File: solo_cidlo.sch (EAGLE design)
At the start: 4 parts, among them Q1 QRD1114

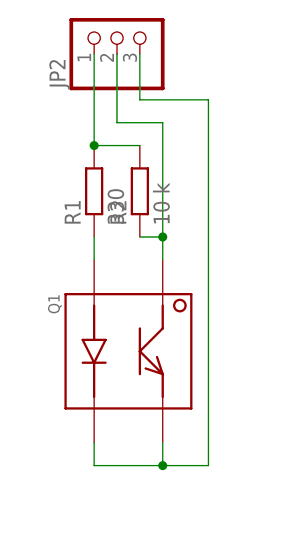
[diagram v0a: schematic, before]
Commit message: Add files via upload
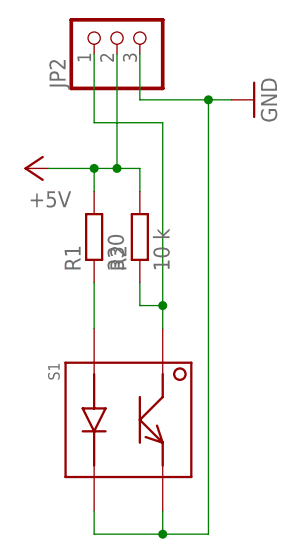
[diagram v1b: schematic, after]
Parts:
- removed Q1: QRD1114, QRD1114:QRD1114
- added S1: QRD1114, QRD1114:QRD1114
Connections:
- removed net N$3: JP2.1, R1.2, R2.2
- removed net N$4: JP2.3, Q1.P$2, Q1.P$4
- new net +5V: JP2.2, R1.2, R2.2
- new net GND: JP2.3, S1.P$2, S1.P$4
- net N$1: now also S1.P$3; no longer Q1.P$3
- net N$2: now also JP2.1, S1.P$1; no longer JP2.2, Q1.P$1
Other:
- moved on the sheet: R1, R2
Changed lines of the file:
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@@
 <layers>
 <layer number="1" name="Top" color="4" fill="1" visible="no" active="no"/>
+<layer number="2" name="Route2" color="1" fill="3" visible="no" active="no"/>
+<layer number="3" name="Route3" color="4" fill="3" visible="no" active="no"/>
+<layer number="4" name="Route4" color="1" fill="4" visible="no" active="no"/>
+<layer number="5" name="Route5" color="4" fill="4" visible="no" active="no"/>
+<layer number="6" name="Route6" color="1" fill="8" visible="no" active="no"/>
+<layer number="7" name="Route7" color="4" fill="8" visible="no" active="no"/>
+<layer number="8" name="Route8" color="1" fill="2" visible="no" active="no"/>
+<layer number="9" name="Route9" color="4" fill="2" visible="no" active="no"/>
+<layer number="10" name="Route10" color="1" fill="7" visible="no" active="no"/>
+<layer number="11" name="Route11" color="4" fill="7" visible="no" active="no"/>
+<layer number="12" name="Route12" color="1" fill="5" visible="no" active="no"/>
+<layer number="13" name="Route13" color="4" fill="5" visible="no" active="no"/>
+<layer number="14" name="Route14" color="1" fill="6" visible="no" active="no"/>
+<layer number="15" name="Route15" color="4" fill="6" visible="no" active="no"/>
 <layer number="16" name="Bottom" color="1" fill="1" visible="no" active="no"/>
 <layer number="17" name="Pads" color="2" fill="1" visible="no" active="no"/>
@@
 </classes>
 <parts>
-<part name="Q1" library="QRD1114" deviceset="QRD1114" device=""/>
+<part name="S1" library="QRD1114" deviceset="QRD1114" device=""/>
 <part name="R1" library="resistor" library_urn="urn:adsk.eagle:library:348" deviceset="R-EU_" device="MELF0102W" package3d_urn="urn:adsk.eagle:package:26105/1" value="330"/>
 <part name="R2" library="resistor" library_urn="urn:adsk.eagle:library:348" deviceset="R-EU_" device="MELF0102W" package3d_urn="urn:adsk.eagle:package:26105/1" value="10 k"/>
 <part name="JP2" library="pinhead" library_urn="urn:adsk.eagle:library:325" deviceset="PINHD-1X3" device="" package3d_urn="urn:adsk.eagle:package:22458/2"/>
+<part name="GND1" library="supply1" library_urn="urn:adsk.eagle:library:371" deviceset="GND" device=""/>
+<part name="P+1" library="supply1" library_urn="urn:adsk.eagle:library:371" deviceset="+5V" device=""/>
 </parts>
 <sheets>
@@
 </plain>
 <instances>
-<instance part="Q1" gate="G$1" x="43.18" y="45.72"/>
-<instance part="R1" gate="G$1" x="40.64" y="63.5" rot="R90"/>
-<instance part="R2" gate="G$1" x="45.72" y="63.5" rot="R90"/>
+<instance part="S1" gate="G$1" x="43.18" y="38.1"/>
+<instance part="R1" gate="G$1" x="40.64" y="58.42" rot="R90"/>
+<instance part="R2" gate="G$1" x="45.72" y="58.42" rot="R90"/>
 <instance part="JP2" gate="A" x="43.18" y="81.28" rot="R90"/>
+<instance part="GND1" gate="1" x="58.42" y="73.66" rot="R90"/>
+<instance part="P+1" gate="1" x="33.02" y="66.04" rot="R90"/>
 </instances>
 <busses>
@@
 <net name="N$1" class="0">
 <segment>
-<pinref part="Q1" gate="G$1" pin="P$3"/>
+<pinref part="S1" gate="G$1" pin="P$3"/>
 <pinref part="R1" gate="G$1" pin="1"/>
-<wire x1="40.64" y1="55.88" x2="40.64" y2="58.42" width="0.1524" layer="91"/>
+<wire x1="40.64" y1="48.26" x2="40.64" y2="53.34" width="0.1524" layer="91"/>
 </segment>
 </net>
 <net name="N$2" class="0">
 <segment>
+<pinref part="S1" gate="G$1" pin="P$1"/>
+<wire x1="48.26" y1="48.26" x2="48.26" y2="50.8" width="0.1524" layer="91"/>
+<wire x1="48.26" y1="50.8" x2="48.26" y2="71.12" width="0.1524" layer="91"/>
 <pinref part="R2" gate="G$1" pin="1"/>
-<wire x1="45.72" y1="58.42" x2="48.26" y2="58.42" width="0.1524" layer="91"/>
-<pinref part="Q1" gate="G$1" pin="P$1"/>
-<wire x1="48.26" y1="58.42" x2="48.26" y2="55.88" width="0.1524" layer="91"/>
-<junction x="48.26" y="58.42"/>
-<wire x1="48.26" y1="58.42" x2="48.26" y2="71.12" width="0.1524" layer="91"/>
-<wire x1="48.26" y1="71.12" x2="43.18" y2="71.12" width="0.1524" layer="91"/>
-<pinref part="JP2" gate="A" pin="2"/>
-<wire x1="43.18" y1="71.12" x2="43.18" y2="78.74" width="0.1524" layer="91"/>
+<wire x1="45.72" y1="53.34" x2="45.72" y2="50.8" width="0.1524" layer="91"/>
+<wire x1="45.72" y1="50.8" x2="48.26" y2="50.8" width="0.1524" layer="91"/>
+<junction x="48.26" y="50.8"/>
+<pinref part="JP2" gate="A" pin="1"/>
+<wire x1="48.26" y1="71.12" x2="40.64" y2="71.12" width="0.1524" layer="91"/>
+<wire x1="40.64" y1="71.12" x2="40.64" y2="78.74" width="0.1524" layer="91"/>
 </segment>
 </net>
-<net name="N$3" class="0">
+<net name="GND" class="0">
 <segment>
-<pinref part="R1" gate="G$1" pin="2"/>
-<pinref part="R2" gate="G$1" pin="2"/>
-<wire x1="40.64" y1="68.58" x2="45.72" y2="68.58" width="0.1524" layer="91"/>
-<junction x="40.64" y="68.58"/>
-<pinref part="JP2" gate="A" pin="1"/>
-<wire x1="40.64" y1="68.58" x2="40.64" y2="78.74" width="0.1524" layer="91"/>
+<pinref part="S1" gate="G$1" pin="P$4"/>
+<wire x1="40.64" y1="27.94" x2="40.64" y2="25.4" width="0.1524" layer="91"/>
+<wire x1="40.64" y1="25.4" x2="48.26" y2="25.4" width="0.1524" layer="91"/>
+<wire x1="48.26" y1="25.4" x2="53.34" y2="25.4" width="0.1524" layer="91"/>
+<wire x1="53.34" y1="25.4" x2="53.34" y2="73.66" width="0.1524" layer="91"/>
+<wire x1="53.34" y1="73.66" x2="45.72" y2="73.66" width="0.1524" layer="91"/>
+<pinref part="S1" gate="G$1" pin="P$2"/>
+<wire x1="48.26" y1="27.94" x2="48.26" y2="25.4" width="0.1524" layer="91"/>
+<junction x="48.26" y="25.4"/>
+<pinref part="JP2" gate="A" pin="3"/>
+<wire x1="45.72" y1="73.66" x2="45.72" y2="78.74" width="0.1524" layer="91"/>
+<pinref part="GND1" gate="1" pin="GND"/>
+<wire x1="55.88" y1="73.66" x2="53.34" y2="73.66" width="0.1524" layer="91"/>
+<junction x="53.34" y="73.66"/>
 </segment>
 </net>
-<net name="N$4" class="0">
+<net name="+5V" class="0">
 <segment>
-<pinref part="Q1" gate="G$1" pin="P$4"/>
-<wire x1="40.64" y1="35.56" x2="40.64" y2="33.02" width="0.1524" layer="91"/>
-<wire x1="40.64" y1="33.02" x2="48.26" y2="33.02" width="0.1524" layer="91"/>
-<wire x1="48.26" y1="33.02" x2="53.34" y2="33.02" width="0.1524" layer="91"/>
-<wire x1="53.34" y1="33.02" x2="53.34" y2="73.66" width="0.1524" layer="91"/>
-<wire x1="53.34" y1="73.66" x2="45.72" y2="73.66" width="0.1524" layer="91"/>
-<pinref part="Q1" gate="G$1" pin="P$2"/>
-<wire x1="48.26" y1="35.56" x2="48.26" y2="33.02" width="0.1524" layer="91"/>
-<junction x="48.26" y="33.02"/>
-<pinref part="JP2" gate="A" pin="3"/>
-<wire x1="45.72" y1="73.66" x2="45.72" y2="78.74" width="0.1524" layer="91"/>
+<pinref part="JP2" gate="A" pin="2"/>
+<wire x1="43.18" y1="78.74" x2="43.18" y2="66.04" width="0.1524" layer="91"/>
+<wire x1="43.18" y1="66.04" x2="45.72" y2="66.04" width="0.1524" layer="91"/>
+<pinref part="R2" gate="G$1" pin="2"/>
+<wire x1="45.72" y1="66.04" x2="45.72" y2="63.5" width="0.1524" layer="91"/>
+<pinref part="R1" gate="G$1" pin="2"/>
+<wire x1="43.18" y1="66.04" x2="40.64" y2="66.04" width="0.1524" layer="91"/>
+<wire x1="40.64" y1="66.04" x2="40.64" y2="63.5" width="0.1524" layer="91"/>
+<junction x="43.18" y="66.04"/>
+<pinref part="P+1" gate="1" pin="+5V"/>
+<wire x1="35.56" y1="66.04" x2="40.64" y2="66.04" width="0.1524" layer="91"/>
+<junction x="40.64" y="66.04"/>
 </segment>
 </net>
